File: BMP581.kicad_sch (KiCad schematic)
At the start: 3 parts, among them U8 BMP581

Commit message: fix lib
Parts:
- removed U8: BMP581, bmp581:QFN10_BMP581_BOS, symbol 2025-10-01_18-19-23:BMP581
- added U8: BMP581, ACS_Footprint_Library:QFN10_BMP581_BOS, symbol ACS_symbol_Library:BMP581
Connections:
- net +3V3: now also U8.1 (VDDIO), U8.10 (VDD)
- net CSB: now also U8.6 (CSB)
- net GND: now also U8.3 (VSS), U8.8 (VSS), U8.9 (VSS)
- net INT: now also U8.7 (INT)
- net MISO: now also U8.5 (SDO)
- net MOSI: now also U8.4 (SDI)
- net SCK: now also U8.2 (SCK)
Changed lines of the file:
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@@
+	)
+	(symbol
+		(lib_id "ACS_symbol_Library:BMP581")
+		(at 144.78 78.74 0)
+		(unit 1)
+		(exclude_from_sim no)
+		(in_bom yes)
+		(on_board yes)
+		(dnp no)
+		(fields_autoplaced yes)
+		(property "Reference" "U8"
+			(at 165.1 68.58 0)
+			(effects
+				(font
+					(size 1.524 1.524)
+				)
+			)
+		)
+		(property "Value" "BMP581"
+			(at 165.1 71.12 0)
+			(effects
+				(font
+					(size 1.524 1.524)
+				)
+			)
+		)
+		(property "Footprint" "ACS_Footprint_Library:QFN10_BMP581_BOS"
+			(at 144.78 78.74 0)
+			(effects
+				(font
+					(size 1.27 1.27)
+					(italic yes)
+				)
+				(hide yes)
+			)
+		)
+		(property "Datasheet" "BMP581"
+			(at 144.78 78.74 0)
+			(effects
+				(font
+					(size 1.27 1.27)
+					(italic yes)
+				)
+				(hide yes)
+			)
+		)
+		(property "Description" ""
+			(at 144.78 78.74 0)
+			(effects
+				(font
+					(size 1.27 1.27)
+				)
+				(hide yes)
+			)
+		)
+		(pin "1"
+		)
+		(pin "6"
+		)
+		(pin "5"
+		)
+		(pin "4"
+		)
+		(pin "2"
+		)
+		(pin "7"
+		)
+		(pin "8"
+		)
+		(pin "9"
+		)
+		(pin "10"
+		)
+		(pin "3"
+		)
+		(instances
+			(project ""
+				(path "/51f244b9-9601-4f29-b08e-b866e02fd2b7/b7f700c5-467d-4631-8bf8-ae557bc42526"
+					(reference "U8")
+					(unit 1)
+				)
+			)
+		)
 	)
 	(symbol
@@
 					(unit 1)
 				)
-			)
-		)
-	)
-	(symbol
-		(lib_id "2025-10-01_18-19-23:BMP581")
-		(at 144.78 78.74 0)
-		(unit 1)
-		(exclude_from_sim no)
-		(in_bom yes)
-		(on_board yes)
-		(dnp no)
-		(fields_autoplaced yes)
-		(property "Reference" "U8"
-			(at 165.1 68.58 0)
-			(effects
-				(font
-					(size 1.524 1.524)
-				)
-			)
-		)
-		(property "Value" "BMP581"
-			(at 165.1 71.12 0)
-			(effects
-				(font
-					(size 1.524 1.524)
-				)
-			)
-		)
-		(property "Footprint" "bmp581:QFN10_BMP581_BOS"
-			(at 144.78 78.74 0)
-			(effects
-				(font
-					(size 1.27 1.27)
-					(italic yes)
-				)
-				(hide yes)
-			)
-		)
-		(property "Datasheet" "BMP581"
-			(at 144.78 78.74 0)
-			(effects
-				(font
-					(size 1.27 1.27)
-					(italic yes)
-				)
-				(hide yes)
-			)
-		)
-		(property "Description" ""
-			(at 144.78 78.74 0)
-			(effects
-				(font
-					(size 1.27 1.27)
-				)
-				(hide yes)
-			)
-		)
-		(pin "5"
-		)
-		(pin "4"
-		)
-		(pin "2"
-		)
-		(pin "6"
-		)
-		(pin "7"
-		)
-		(pin "8"
-		)
-		(pin "9"
-		)
-		(pin "10"
-		)
-		(pin "1"
-		)
-		(pin "3"
-		)
-		(instances
-			(project ""
-				(path "/51f244b9-9601-4f29-b08e-b866e02fd2b7/b7f700c5-467d-4631-8bf8-ae557bc42526"
-					(reference "U8")
-					(unit 1)
-				)

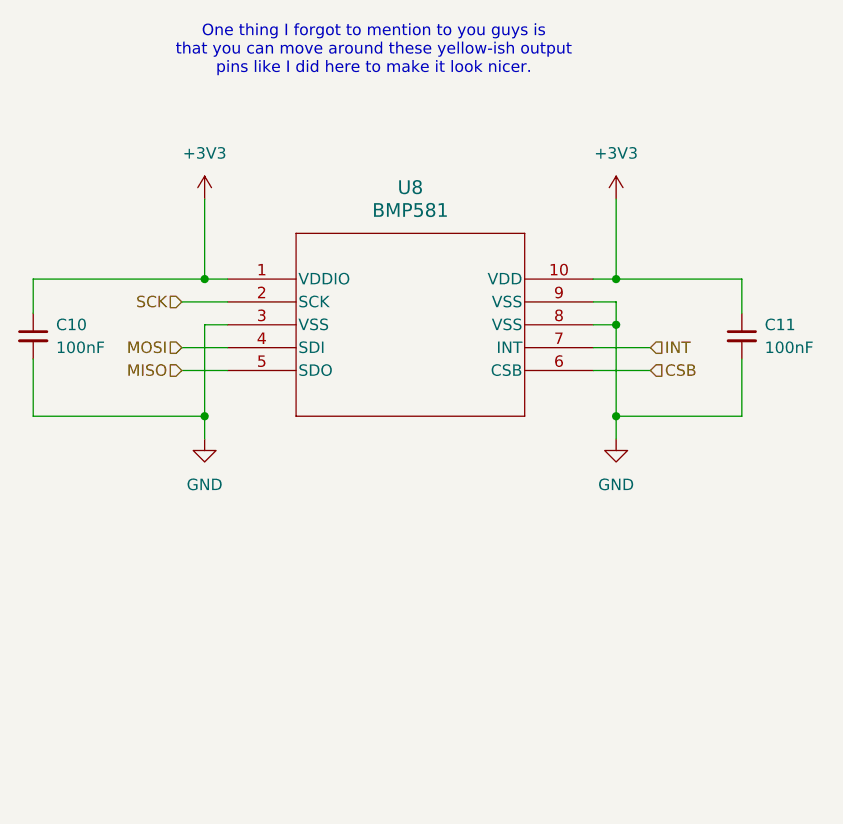
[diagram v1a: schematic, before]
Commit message: lots
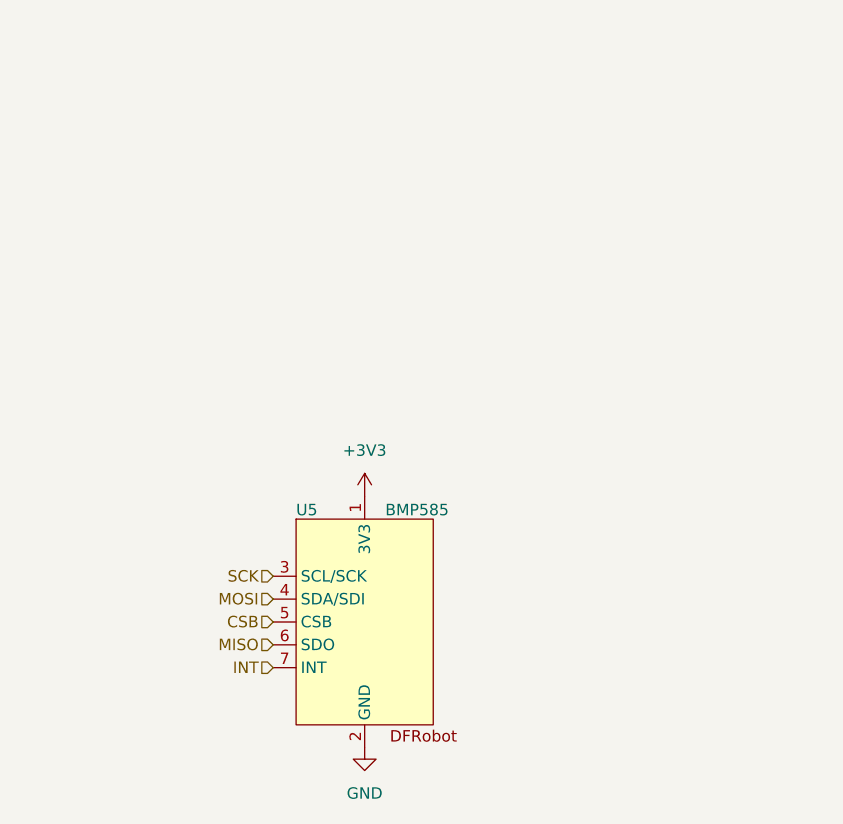
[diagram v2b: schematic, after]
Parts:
- removed C10, C11: 100nF, Capacitor_SMD:C_0603_1608Metric, symbol Device:C_Small
- removed U8: BMP581, ACS_Footprint_Library:QFN10_BMP581_BOS, symbol ACS_symbol_Library:BMP581
- added U5: BMP585, Sensor_Pressure:DFRobot BMP585, symbol Sensor_Pressure:DFRobot_BMP585
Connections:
- net +3V3: now also U5.1 (3V3)
- net CSB: now also U5.5 (CSB)
- net GND: now also U5.2 (GND)
- net INT: now also U5.7 (INT)
- net MISO: now also U5.6 (SDO)
- net MOSI: now also U5.4 (SDA/SDI)
- net SCK: now also U5.3 (SCL/SCK)
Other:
- note removed: "One thing I forgot to mention to you guys is that you can move around these yellow-ish output pins like I did here to make it look nicer."
